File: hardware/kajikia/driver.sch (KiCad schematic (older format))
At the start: 0 parts

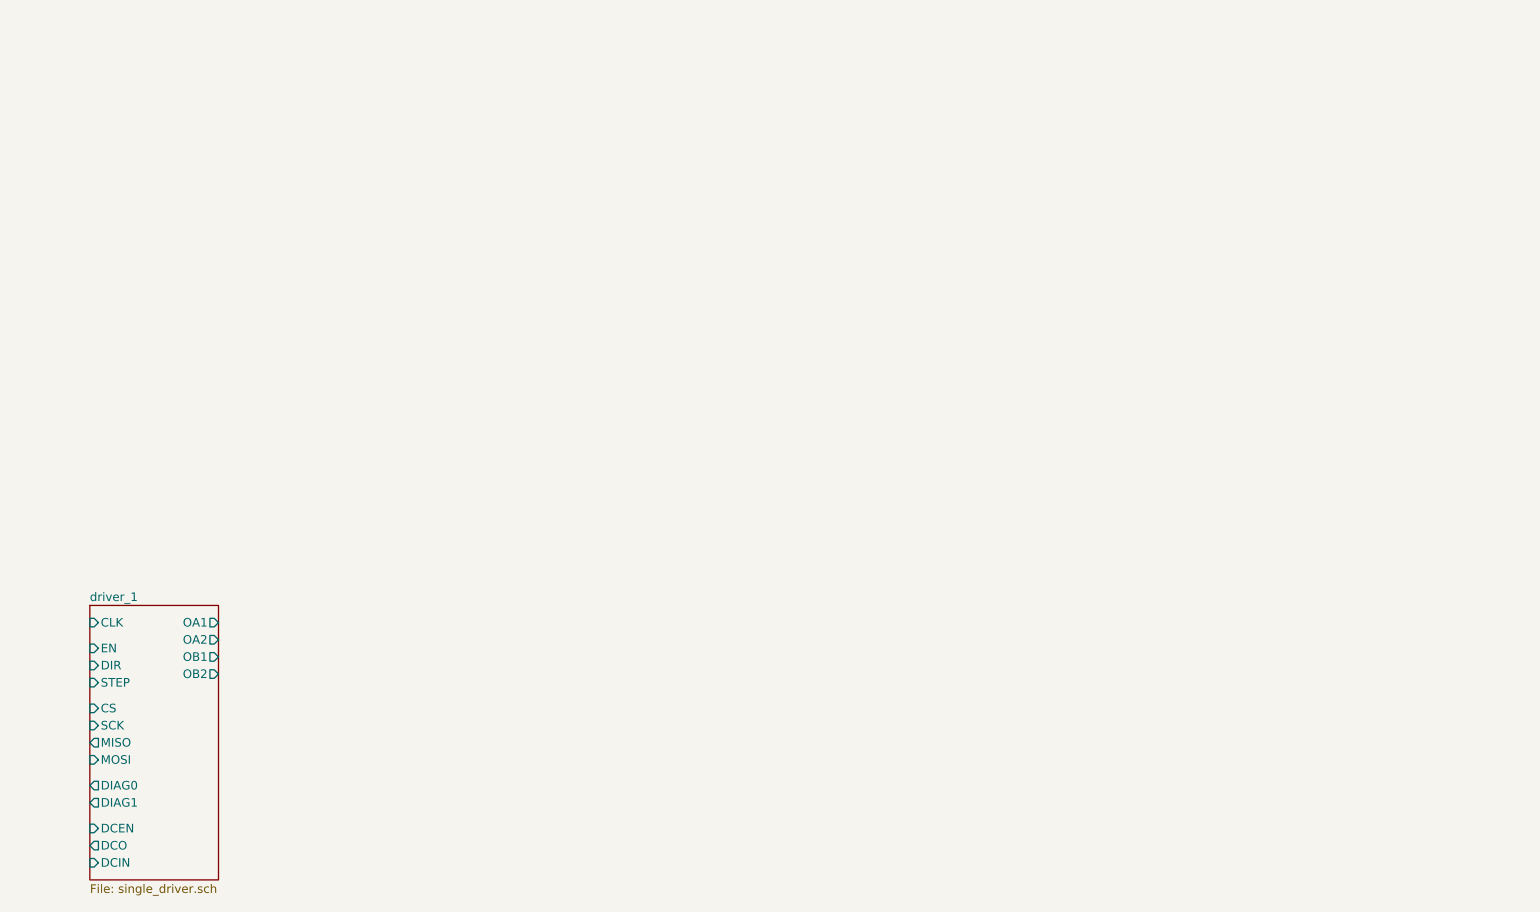
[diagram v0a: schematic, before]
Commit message: io assignments
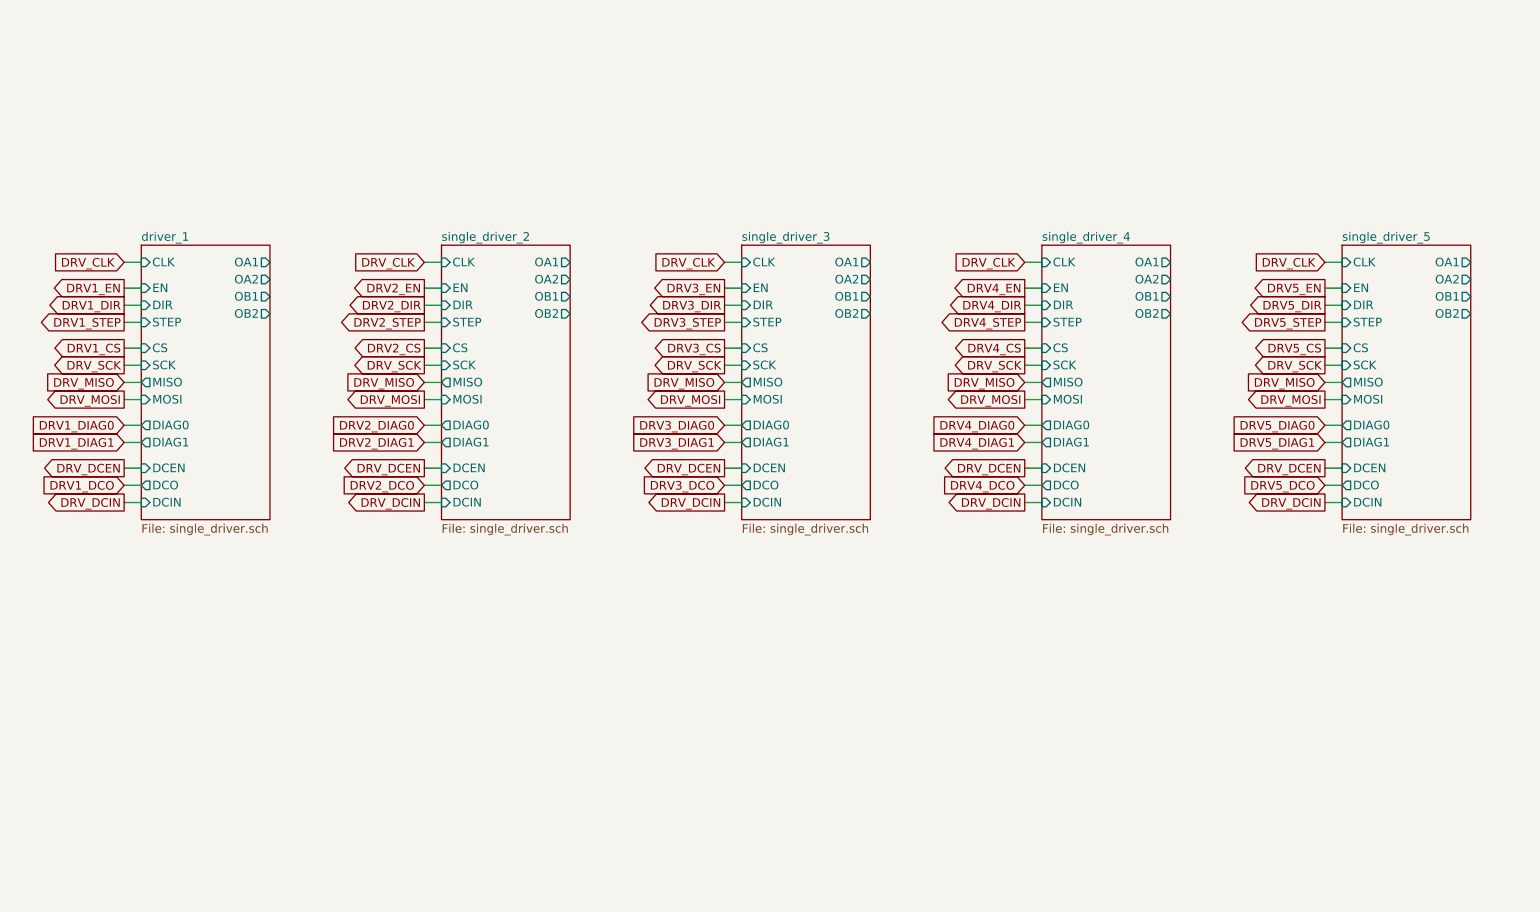
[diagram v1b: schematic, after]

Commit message: io assignments
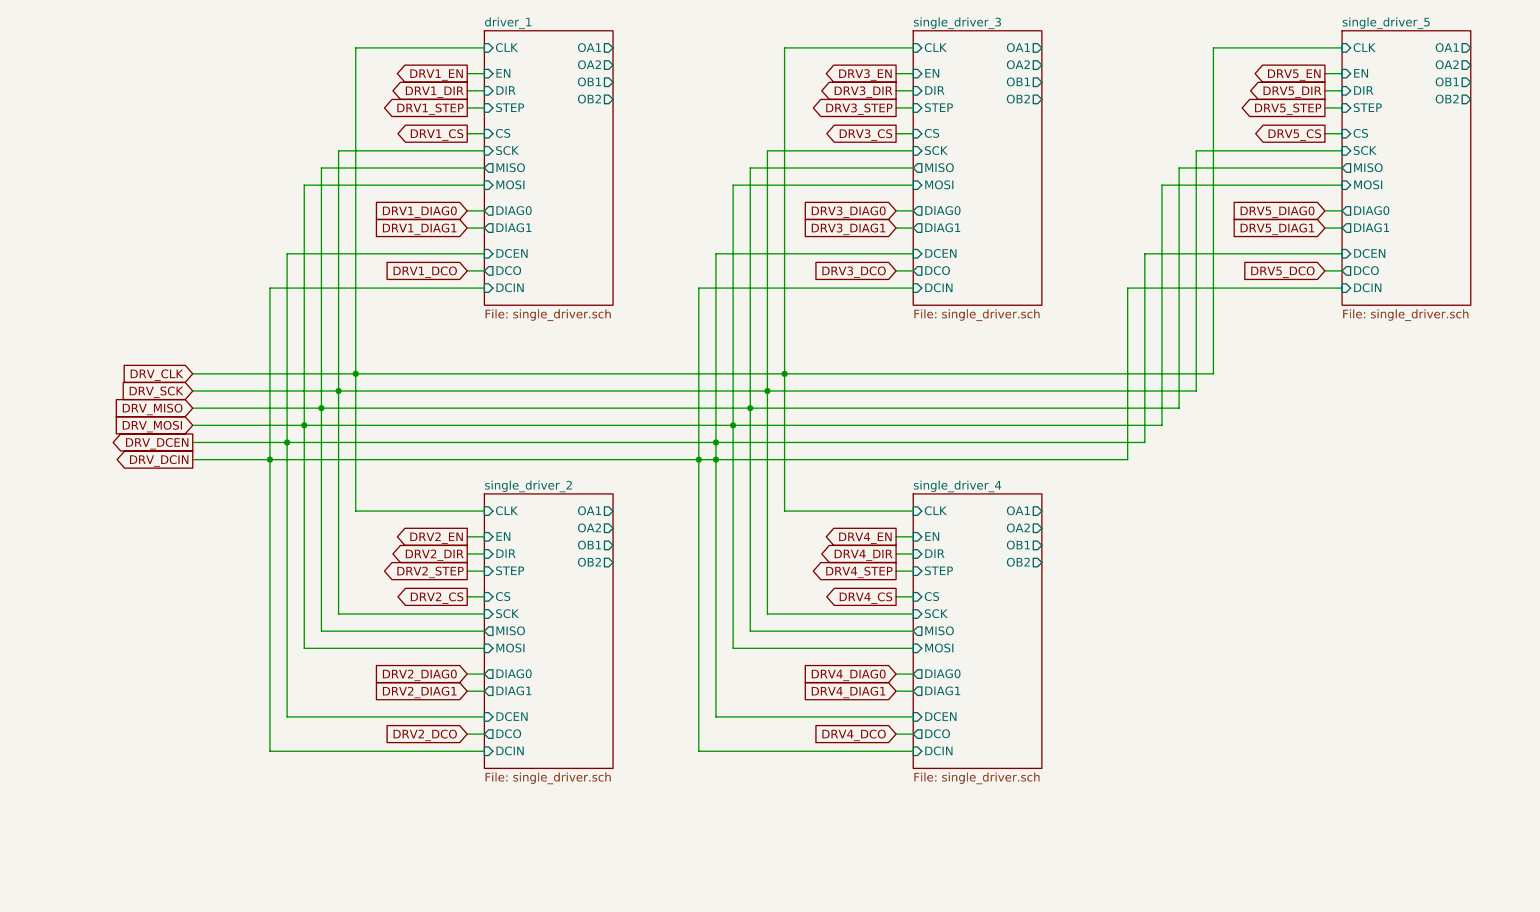
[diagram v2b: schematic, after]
